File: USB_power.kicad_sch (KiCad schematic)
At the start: 20 parts, among them J1 PWR_IN, J2 USB_A_Stacked, J3 Power_check, J4 USB_C_Receptacle_USB2.0_16P

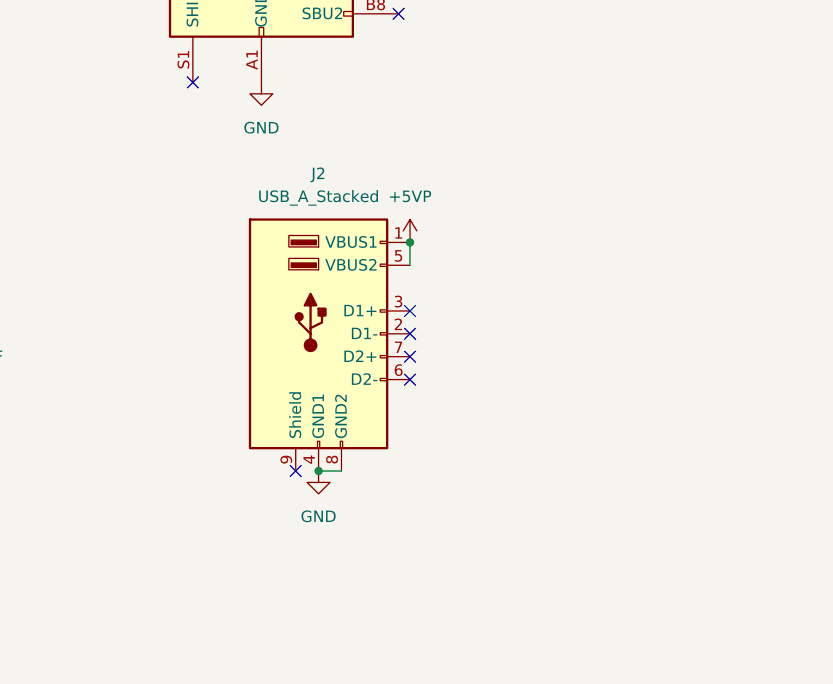
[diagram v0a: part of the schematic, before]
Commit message: 穴あけなど
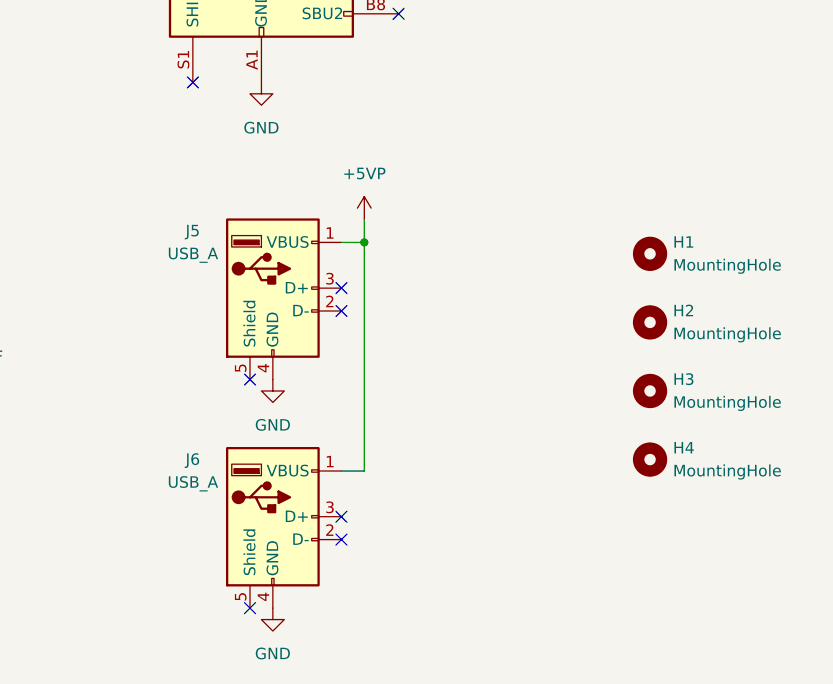
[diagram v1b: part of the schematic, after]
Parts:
- removed J2: USB_A_Stacked, Connector_USB:USB_A_CUI_UJ2-ADH-TH_Horizontal_Stacked, symbol Connector:USB_A_Stacked
- added H1, H2, H3, H4: MountingHole, MountingHole:MountingHole_3.2mm_M3, symbol Mechanical:MountingHole
- added J5, J6: USB_A, Connector_USB:USB_A_CONNFLY_DS1095-WNR0, symbol Connector:USB_A
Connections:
- net +5VP: now also J5.1 (VBUS), J6.1 (VBUS)
- net GND: now also J5.4 (GND), J6.4 (GND)
- no-connect marks 24 -> 25
